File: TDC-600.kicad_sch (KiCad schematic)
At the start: 32 parts, among them J1 MSXCART1, J2 Conn_01x03_Male, J3 Conn_01x03_Male, J4 Conn_01x03_Male, J5 Conn_01x03_Male, J6 FDD Connector, J7 ROM_SWITCH, SW1 SW_Push, U1 AT28C256, U2 74LS04, U3 74LS138, U4 WDC37C65, Y1 16Mhz

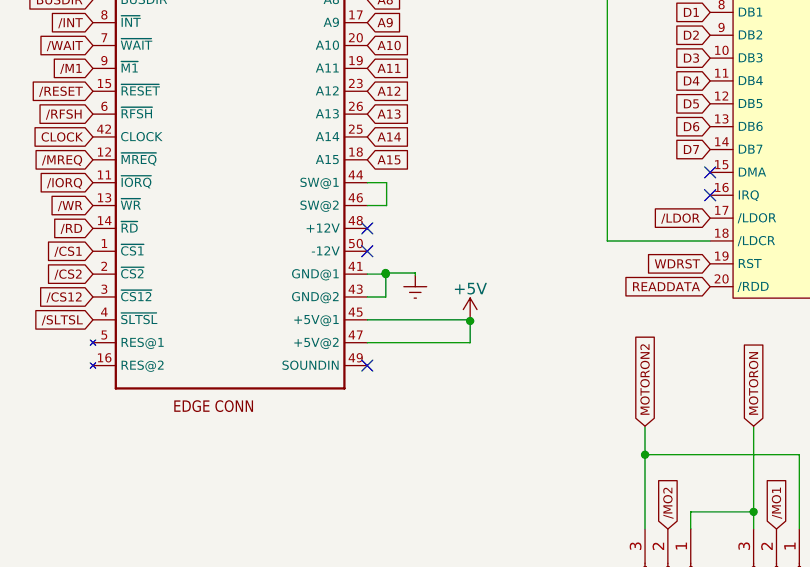
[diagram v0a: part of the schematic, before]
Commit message: Routing Release 1.0
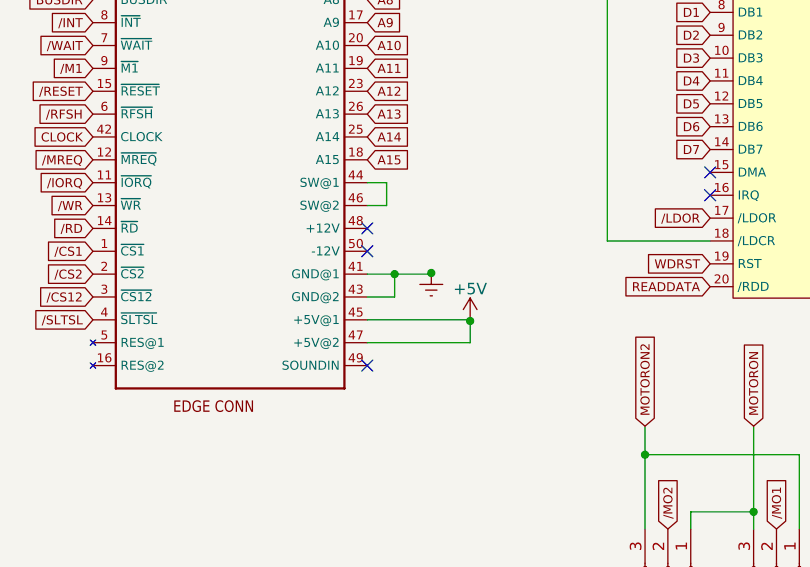
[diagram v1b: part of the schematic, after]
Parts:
- J1: footprint Roni Footprints:MSX_CART_SW_Official_3Holes -> Roni_Footprints:MSX_CART_SW_Official
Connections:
- net GNDREF: now also J1.41 (GND@1), J1.43 (GND@2)
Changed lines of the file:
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@@
   (junction (at 203.581 92.71) (diameter 0) (color 0 0 0 0)
   )
-  (junction (at 60.9838 78.867) (diameter 0) (color 0 0 0 0)
+  (junction (at 61.9643 78.867) (diameter 0) (color 0 0 0 0)
   )
   (junction (at 193.04 66.294) (diameter 0) (color 0 0 0 0)
@@
   (junction (at 193.04 71.374) (diameter 0) (color 0 0 0 0)
   )
+  (junction (at 66.04 78.74) (diameter 0) (color 0 0 0 0)
+  )
   (junction (at 228.346 125.857) (diameter 0) (color 0 0 0 0)
   )
@@
   )
   (junction (at 70.358 84.074) (diameter 0) (color 0 0 0 0)
-  )
-  (junction (at 60.96 78.74) (diameter 0) (color 0 0 0 0)
   )
   (junction (at 85.598 42.164) (diameter 0) (color 0 0 0 0)
@@
     (stroke (width 0) (type default) (color 0 0 0 0))
   )
-  (wire (pts (xy 58.928 78.867) (xy 60.9838 78.867))
-    (stroke (width 0) (type default) (color 0 0 0 0))
-  )
   (wire (pts (xy 129.286 105.664) (xy 121.666 105.664))
     (stroke (width 0) (type default) (color 0 0 0 0))
@@
     (stroke (width 0) (type default) (color 0 0 0 0))
   )
-  (wire (pts (xy 58.928 81.407) (xy 60.9838 81.407))
+  (wire (pts (xy 58.928 81.407) (xy 61.9643 81.407))
+    (stroke (width 0) (type default) (color 0 0 0 0))
+  )
+  (wire (pts (xy 66.04 78.867) (xy 66.04 78.74))
     (stroke (width 0) (type default) (color 0 0 0 0))
   )
@@
     (stroke (width 0) (type default) (color 0 0 0 0))
   )
-  (wire (pts (xy 60.9838 81.407) (xy 60.9838 78.867))
+  (wire (pts (xy 58.928 78.867) (xy 61.9643 78.867))
     (stroke (width 0) (type default) (color 0 0 0 0))
   )
@@
     (stroke (width 0) (type default) (color 0 0 0 0))
   )
+  (wire (pts (xy 61.9643 81.407) (xy 61.9643 78.867))
+    (stroke (width 0) (type default) (color 0 0 0 0))
+  )
   (wire (pts (xy 215.392 125.857) (xy 220.345 125.857))
     (stroke (width 0) (type default) (color 0 0 0 0))
@@
     (stroke (width 0) (type default) (color 0 0 0 0))
   )
+  (wire (pts (xy 61.9643 78.867) (xy 66.04 78.867))
+    (stroke (width 0) (type default) (color 0 0 0 0))
+  )
   (wire (pts (xy 165.354 145.161) (xy 178.054 145.161))
     (stroke (width 0) (type default) (color 0 0 0 0))
@@
     (stroke (width 0) (type default) (color 0 0 0 0))
   )
-  (wire (pts (xy 64.262 78.74) (xy 64.262 78.994))
-    (stroke (width 0) (type default) (color 0 0 0 0))
-  )
   (wire (pts (xy 122.174 132.588) (xy 122.174 130.048))
     (stroke (width 0) (type default) (color 0 0 0 0))
@@
   )
   (wire (pts (xy 108.204 137.668) (xy 109.474 137.668))
-    (stroke (width 0) (type default) (color 0 0 0 0))
-  )
-  (wire (pts (xy 60.96 78.74) (xy 64.262 78.74))
     (stroke (width 0) (type default) (color 0 0 0 0))
   )
@@
     (pin "1")
   )
-  (symbol (lib_id "power:GNDREF") (at 64.262 78.994 0) (unit 1)
-    (in_bom yes) (on_board yes) (fields_autoplaced)
-    (property "Reference" "#PWR01" (id 0) (at 64.262 85.344 0)
-      (effects (font (size 1 1)) hide)
-    )
-    (property "Value" "GNDREF" (id 1) (at 64.262 84.582 0)
-      (effects (font (size 1 1)) hide)
-    )
-    (property "Footprint" "" (id 2) (at 64.262 78.994 0)
-      (effects (font (size 1 1)) hide)
-    )
-    (property "Datasheet" "" (id 3) (at 64.262 78.994 0)
-      (effects (font (size 1 1)) hide)
-    )
-    (pin "1")
-  )
   (symbol (lib_id "power:GNDREF") (at 167.386 83.058 0) (unit 1)
     (in_bom yes) (on_board yes) (fields_autoplaced)
@@
       (effects (font (size 1 1)) hide)
     )
-    (property "Footprint" "Roni Footprints:MSX_CART_SW_Official_3Holes" (id 2) (at 43.688 58.547 0)
+    (property "Footprint" "Roni_Footprints:MSX_CART_SW_Official" (id 2) (at 43.688 58.547 0)
       (effects (font (size 1 1)) hide)
     )
@@
     (pin "7")
   )
+  (symbol (lib_id "power:GNDREF") (at 66.04 78.74 0) (unit 1)
+    (in_bom yes) (on_board yes) (fields_autoplaced)
+    (property "Reference" "#PWR?" (id 0) (at 66.04 85.09 0)
+      (effects (font (size 1 1)) hide)
+    )
+    (property "Value" "GNDREF" (id 1) (at 66.04 84.328 0)
+      (effects (font (size 1 1)) hide)
+    )
+    (property "Footprint" "" (id 2) (at 66.04 78.74 0)
+      (effects (font (size 1 1)) hide)
+    )
+    (property "Datasheet" "" (id 3) (at 66.04 78.74 0)
+      (effects (font (size 1 1)) hide)
+    )
+    (pin "1")
+  )
   (symbol (lib_id "74xx:74LS04") (at 251.206 50.8 0) (unit 1)
     (in_bom yes) (on_board yes)
@@
   )
   (symbol_instances
-    (path "/5fd49dc5-3ef7-42c3-ba98-39fb50cf0473"
-      (reference "#PWR01") (unit 1) (value "GNDREF") (footprint "")
-    )
     (path "/64de7322-3492-44c0-b600-8a8a1cbeb091"
       (reference "#PWR02") (unit 1) (value "+5V") (footprint "")
@@
       (reference "#PWR021") (unit 1) (value "+5V") (footprint "")
     )
+    (path "/f82b494c-be8d-4f2a-a5d0-8b689b314ae2"
+      (reference "#PWR?") (unit 1) (value "GNDREF") (footprint "")
+    )
     (path "/b16493d0-17e8-4588-8dc9-b6b9eb468398"
       (reference "C1") (unit 1) (value "10uF") (footprint "Capacitor_THT:CP_Radial_D4.0mm_P1.50mm")
@@
     )
     (path "/c88d69e7-0f10-442f-b4e9-d3ac6c8cb585"
-      (reference "J1") (unit 1) (value "MSXCART1") (footprint "Roni Footprints:MSX_CART_SW_Official_3Holes")
+      (reference "J1") (unit 1) (value "MSXCART1") (footprint "Roni_Footprints:MSX_CART_SW_Official")
     )
     (path "/3712ef9a-3384-4ffe-bc7d-57032448a0fc"
